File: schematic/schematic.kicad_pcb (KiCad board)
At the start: 2 copper layers, 99.1 x 99.1 mm, 89 parts, among them J2 USB_C_Receptacle_USB2.0, J3 Peltier Connection, J4 Serial, SW1 Power Switch, U1 ESP32-D-WD-V3, U10 BSD316, U11 BSD316, U12 PC817, U13 PC817, U14 PC817, U15 AS431, U16 LM324, U17 XL6009, U18 PAM2305CGFADJ, U2 PC817, U3 BUK9K52-60E, U4 BUK9K52-60E, U5 LM324, U6 PC817, U7 PC817, U8 PC817, U9 BSD316, Y1 Crystal_GND24

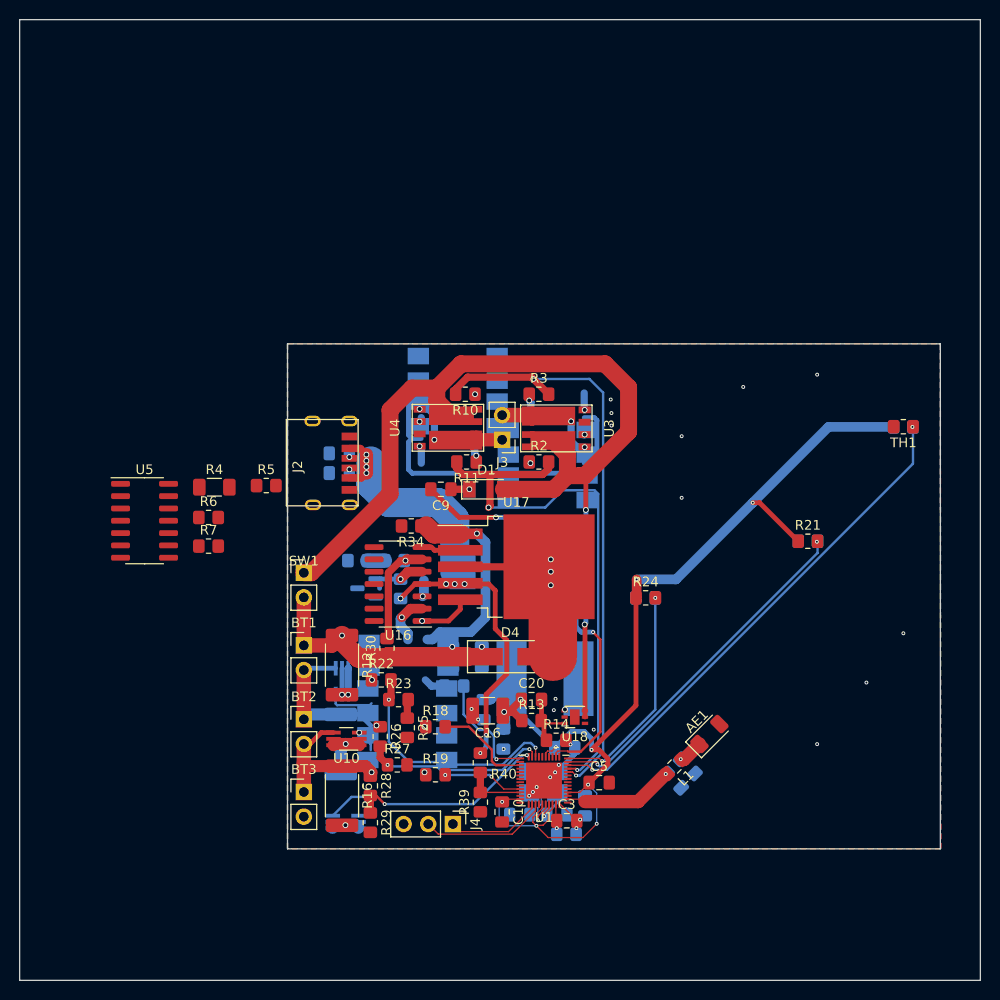
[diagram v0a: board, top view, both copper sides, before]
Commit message: d
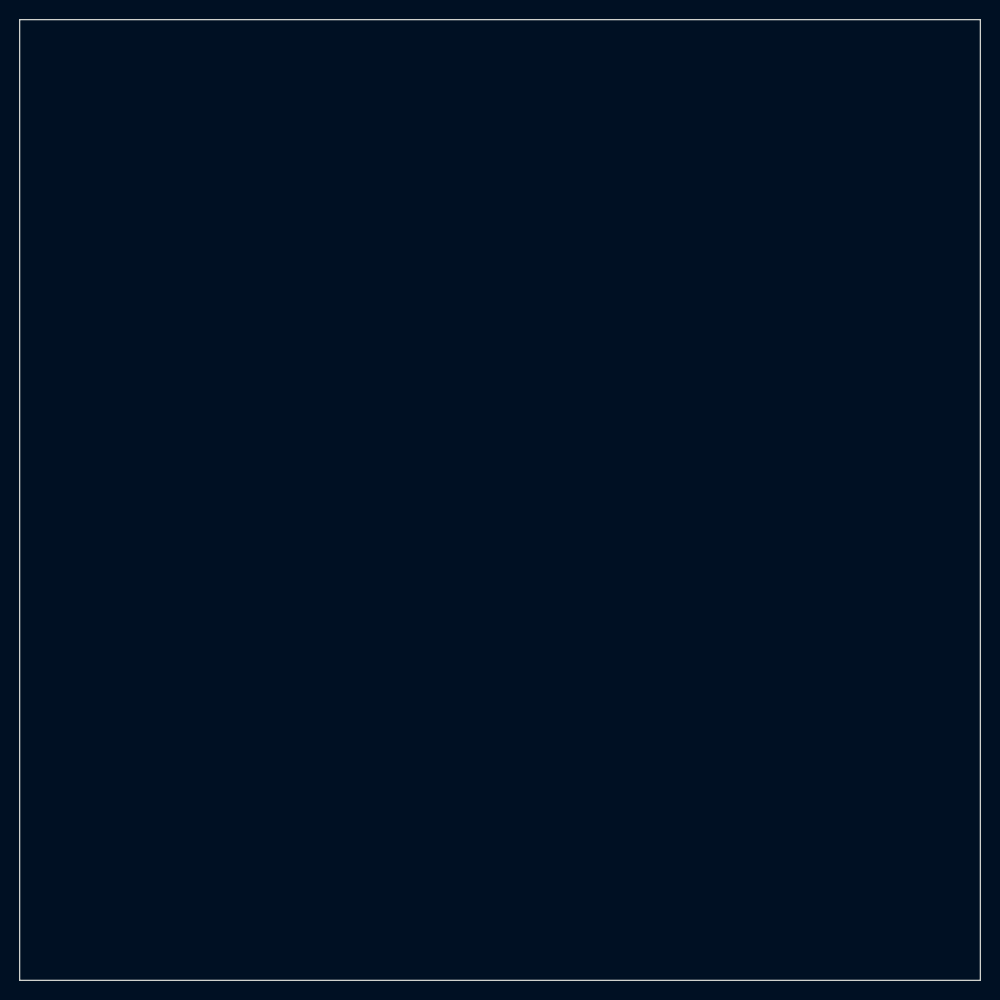
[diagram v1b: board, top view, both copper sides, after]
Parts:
- removed AE1: Antenna_Chip, RF_Antenna:Johanson_2450AT18x100
- removed BT1, BT2, BT3: Battery_Cell, Connector_PinHeader_2.54mm:PinHeader_1x02_P2.54mm_Vertical
- removed C1: 3.797pF, Capacitor_SMD:C_0805_2012Metric_Pad1.18x1.45mm_HandSolder
- removed C10, C21, C5, C8: 100nF, Capacitor_SMD:C_0805_2012Metric_Pad1.18x1.45mm_HandSolder
- removed C11, C15, C17, C9: 10uF, Capacitor_SMD:C_0805_2012Metric_Pad1.18x1.45mm_HandSolder
- removed C16: 100uF, Capacitor_SMD:C_1210_3225Metric_Pad1.33x2.70mm_HandSolder
- removed C18: 1uF, Capacitor_SMD:C_0805_2012Metric_Pad1.18x1.45mm_HandSolder
- removed C2: 4.64pF, Capacitor_SMD:C_0805_2012Metric_Pad1.18x1.45mm_HandSolder
- removed C20: Cfw (DNP), Capacitor_SMD:C_0805_2012Metric_Pad1.18x1.45mm_HandSolder
- removed C3: 3.3nF, Capacitor_SMD:C_0805_2012Metric_Pad1.18x1.45mm_HandSolder
- removed C4: 10nF, Capacitor_SMD:C_0805_2012Metric_Pad1.18x1.45mm_HandSolder
- removed C6, C7: 10pF, Capacitor_SMD:C_0805_2012Metric_Pad1.18x1.45mm_HandSolder
- removed D1, D2: LL4148, Diode_SMD:D_MiniMELF
- removed D4: SS34, Diode_SMD:D_SMA_Handsoldering
- removed J2: USB_C_Receptacle_USB2.0, 1KicadLib:USB4125-GF-A
- removed J3: Peltier Connection, Connector_PinHeader_2.54mm:PinHeader_1x02_P2.54mm_Vertical
- removed J4: Serial, Connector_PinHeader_2.54mm:PinHeader_1x03_P2.54mm_Vertical
- removed L1: 1.807nH, Inductor_SMD:L_0805_2012Metric_Pad1.15x1.40mm_HandSolder
- removed L2: 10uH NR8040T100M, Inductor_SMD:L_Taiyo-Yuden_NR-80xx_HandSoldering
- removed L3: 33uH, Inductor_SMD:L_10.4x10.4_H4.8
- removed R1: 20k, Resistor_SMD:R_0805_2012Metric_Pad1.20x1.40mm_HandSolder
- removed R10, R11, R2, R3: 300, Resistor_SMD:R_0805_2012Metric_Pad1.20x1.40mm_HandSolder
- removed R12, R15, R16: 28.7, Resistor_SMD:R_2512_6332Metric_Pad1.40x3.35mm_HandSolder
- removed R13: 33k, Resistor_SMD:R_0805_2012Metric_Pad1.20x1.40mm_HandSolder
- removed R14: 7.5k, Resistor_SMD:R_0805_2012Metric_Pad1.20x1.40mm_HandSolder
- removed R17, R18, R19: 200, Resistor_SMD:R_0805_2012Metric_Pad1.20x1.40mm_HandSolder
- removed R20, R21, R24: 90k, Resistor_SMD:R_0805_2012Metric_Pad1.20x1.40mm_HandSolder
- removed R22, R40: 100k, Resistor_SMD:R_0805_2012Metric_Pad1.20x1.40mm_HandSolder
- removed R23: 22k, Resistor_SMD:R_0805_2012Metric_Pad1.20x1.40mm_HandSolder
- removed R25: 390, Resistor_SMD:R_0805_2012Metric_Pad1.20x1.40mm_HandSolder
- removed R26: 180k, Resistor_SMD:R_0805_2012Metric_Pad1.20x1.40mm_HandSolder
- removed R27, R29: 68k, Resistor_SMD:R_0805_2012Metric_Pad1.20x1.40mm_HandSolder
- removed R28, R31: 56k, Resistor_SMD:R_0805_2012Metric_Pad1.20x1.40mm_HandSolder
- removed R30: 220k, Resistor_SMD:R_0805_2012Metric_Pad1.20x1.40mm_HandSolder
- removed R32: 120, Resistor_SMD:R_0805_2012Metric_Pad1.20x1.40mm_HandSolder
- removed R33: 500, Resistor_SMD:R_0805_2012Metric_Pad1.20x1.40mm_HandSolder
- removed R34, R7: 12.5k, Resistor_SMD:R_0805_2012Metric_Pad1.20x1.40mm_HandSolder
- removed R39: 150k, Resistor_SMD:R_0805_2012Metric_Pad1.20x1.40mm_HandSolder
- removed R4: .1, Resistor_SMD:R_1206_3216Metric_Pad1.30x1.75mm_HandSolder
- removed R5, R6: 1k, Resistor_SMD:R_0805_2012Metric_Pad1.20x1.40mm_HandSolder
- removed R8, R9: 5.1k, Capacitor_SMD:C_0805_2012Metric_Pad1.18x1.45mm_HandSolder
- removed SW1: Power Switch, Connector_PinHeader_2.54mm:PinHeader_1x02_P2.54mm_Vertical
- removed TH1, TH2, TH3: SDNT2012X103F3950FTF, Resistor_SMD:R_0805_2012Metric_Pad1.20x1.40mm_HandSolder
- removed U1: ESP32-D-WD-V3, Package_DFN_QFN:QFN-48-1EP_5x5mm_P0.35mm_EP3.7x3.7mm
- removed U10, U11, U9: BSD316, Package_TO_SOT_SMD:SOT-363_SC-70-6_Handsoldering
- removed U12, U13, U14, U2, U6, U7, U8: PC817, 1KicadLib:SMT_4_8.2x2.54
- removed U15: AS431, Package_TO_SOT_SMD:SOT-23
- removed U16, U5: LM324, Package_SO:SOIC-14_3.9x8.7mm_P1.27mm
- removed U17: XL6009, Package_TO_SOT_SMD:TO-263-5_TabPin3
- removed U18: PAM2305CGFADJ, Package_DFN_QFN:DFN-6-1EP_2x2mm_P0.65mm_EP1x1.6mm
- removed U3, U4: BUK9K52-60E, 1KicadLib:LFPAK56D
- removed Y1: Crystal_GND24, Crystal:Crystal_SMD_SeikoEpson_FA238-4Pin_3.2x2.5mm_HandSoldering
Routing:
- net VCC_UNREGULATED: track 214.1 -> 0.00 mm, vias 10 -> 0
- net +3V3: track 117.4 -> 0.00 mm, vias 10 -> 0
- net DRIVER_N: track 61.0 -> 0.00 mm, vias 2 -> 0
- net VBUS: track 54.7 -> 0.00 mm, vias 10 -> 0
- net TEMP_SENSE_1: track 52.7 -> 0.00 mm, vias 2 -> 0
- net +BATT: track 51.0 -> 0.00 mm, vias 5 -> 0
- net PWM: track 44.9 -> 0.00 mm, vias 2 -> 0
- net CELL_MEAS_3: track 43.7 -> 0.00 mm, vias 4 -> 0
- net TEMP_SENSE_2: track 36.3 -> 0.00 mm, vias 2 -> 0
- net Net-(BT1-Pad2): track 23.2 -> 0.00 mm, vias 2 -> 0
- net TEMP_SENSE_3: track 22.9 -> 0.00 mm, vias 2 -> 0
- net CELL_MEAS_1: track 20.6 -> 0.00 mm, vias 2 -> 0
- net Net-(D4-Pad2): track 18.6 -> 0.00 mm, vias 3 -> 0
- net Net-(BT2-Pad2): track 15.8 -> 0.00 mm, vias 1 -> 0
- net TXD: track 13.2 -> 0.00 mm
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- removed copper zone on B.Cu, net GND
- removed copper zone on F.Cu, net GND
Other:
- outline, holes or cut-outs redrawn
- board text removed: "GUANTANAMO BAY"
- board text removed: "Joesphan Lu"
